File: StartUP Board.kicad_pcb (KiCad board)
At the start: 2 copper layers, 85.8 x 55 mm, 22 parts, among them IC1 AP7380-33W5-7, J1 Conn_01x05_Socket, U1 ANT13SECQE, U2 CD4049UBDR

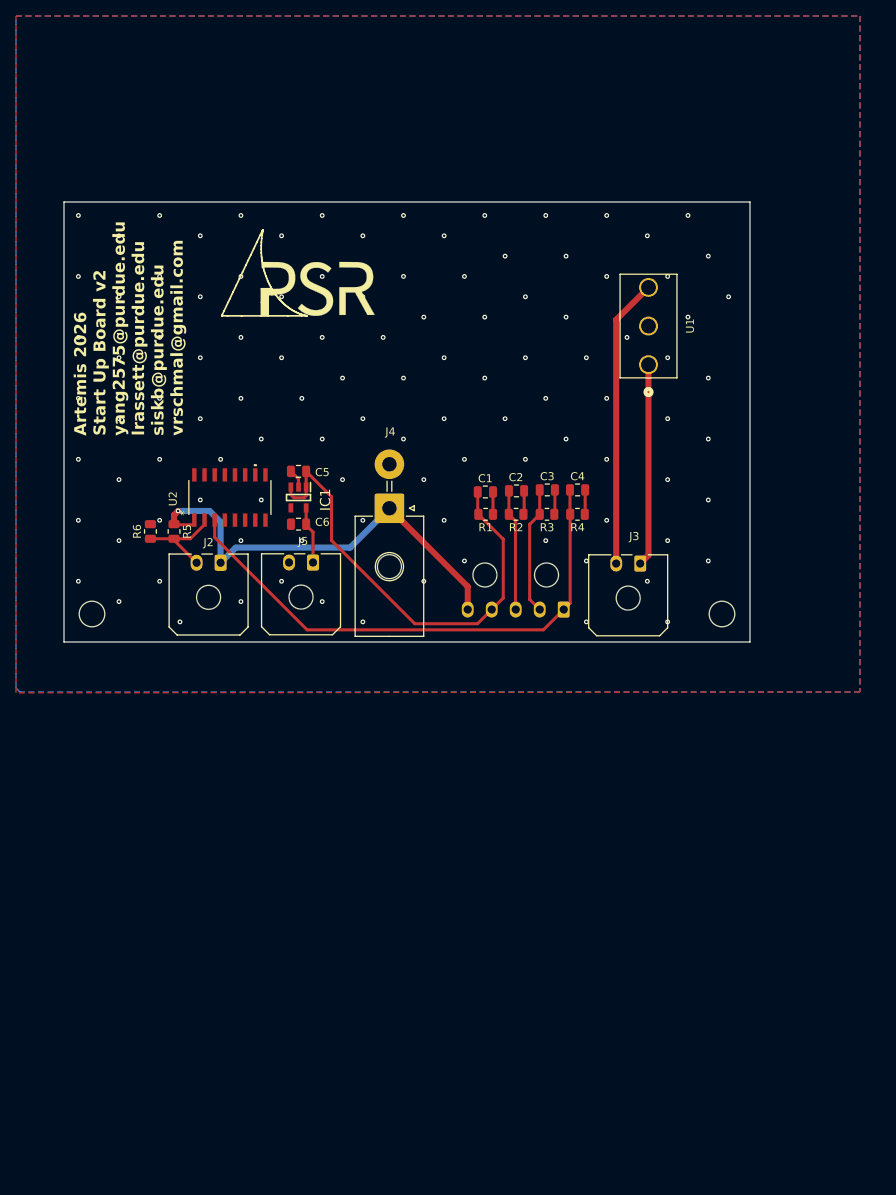
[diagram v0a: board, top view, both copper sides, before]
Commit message: furdue
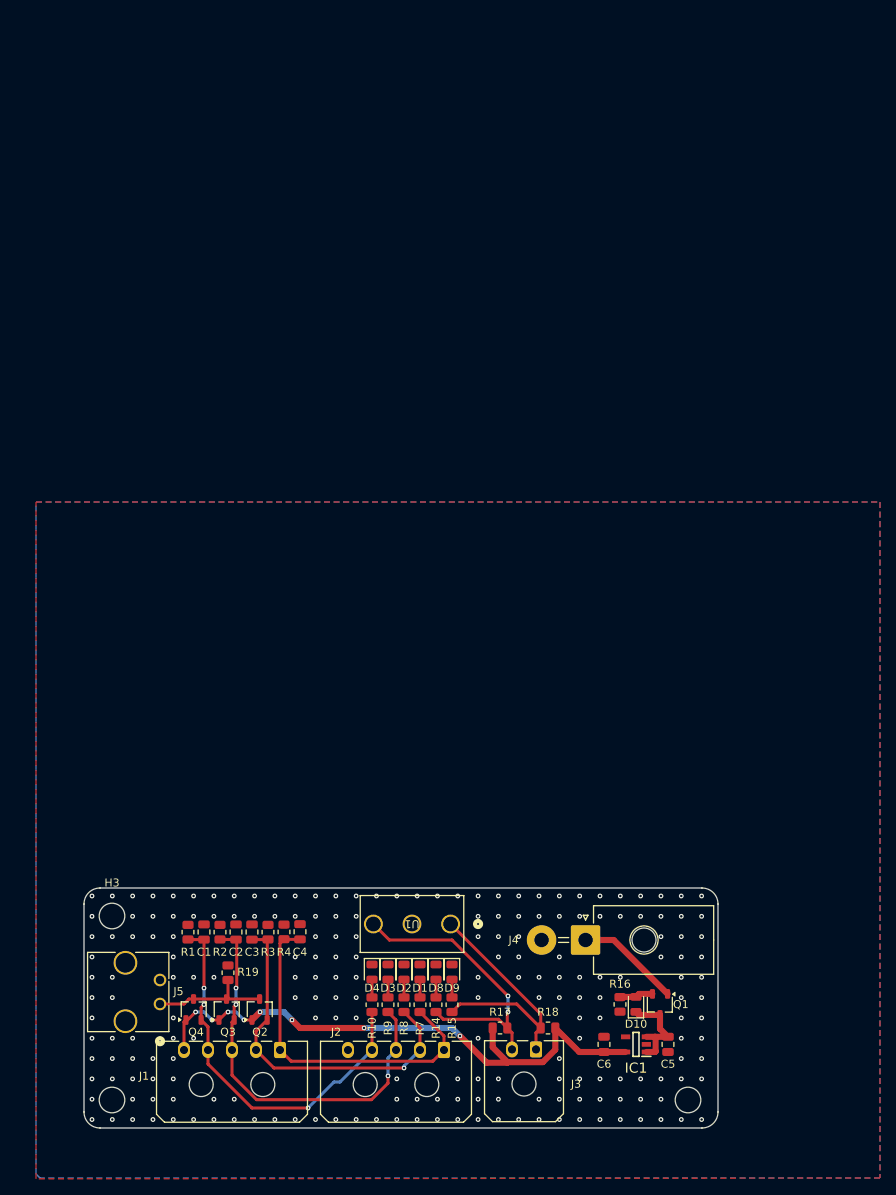
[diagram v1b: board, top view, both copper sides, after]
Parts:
- removed R5, R6: 100k, Resistor_SMD:R_0805_2012Metric
- removed U2: CD4049UBDR, CD4049UBDR:D16-M
- added D1: LED, LED_SMD:LED_0805_2012Metric, F.Cu at (166.0, 105.0)
- added D10: D_Zener, Diode_SMD:D_0805_2012Metric, F.Cu at (193.0, 109.0)
- added D2: LED, LED_SMD:LED_0805_2012Metric, F.Cu at (164.0, 105.0)
- added D3: LED, LED_SMD:LED_0805_2012Metric, F.Cu at (162.0, 105.0)
- added D4: LED, LED_SMD:LED_0805_2012Metric, F.Cu at (160.0, 105.0)
- added D8: LED, LED_SMD:LED_0805_2012Metric, F.Cu at (168.0, 105.0)
- added D9: LED, LED_SMD:LED_0805_2012Metric, F.Cu at (170.0, 105.0)
- added G***: LOGO, LOGO, B.Cu at (172.5, 106.0)
- added G***: LOGO, LOGO, B.Cu at (152.0, 107.5)
- added G***: LOGO, LOGO, B.Cu at (188.3, 108.1)
- added H3: MountingHole, MountingHole:MountingHole_3.2mm_M3, F.Cu at (127.5, 98.0)
- added Q1: PMOS, Package_TO_SOT_SMD:TSOT-23, F.Cu at (196.0, 109.0)
- added Q2: NMOS, Package_TO_SOT_SMD:TSOT-23, F.Cu at (145.9, 109.7)
- added Q3: NMOS, Package_TO_SOT_SMD:TSOT-23, F.Cu at (141.8, 109.7)
- added Q4: NMOS, Package_TO_SOT_SMD:TSOT-23, F.Cu at (137.7, 109.7)
- added R10: 680, Resistor_SMD:R_0805_2012Metric, F.Cu at (160.0, 109.1)
- added R14: 680, Resistor_SMD:R_0805_2012Metric, F.Cu at (168.0, 109.1)
- added R15: 680, Resistor_SMD:R_0805_2012Metric, F.Cu at (170.0, 109.1)
- added R16: 100k, Resistor_SMD:R_0805_2012Metric, F.Cu at (191.0, 109.0)
- added R17: 4.7k, Resistor_SMD:R_0805_2012Metric, F.Cu at (176.0, 112.0)
- added R18: 4.7k, Resistor_SMD:R_0805_2012Metric, F.Cu at (182.0, 112.0)
- added R19: 4.7k, Resistor_SMD:R_0805_2012Metric, F.Cu at (142.0, 105.1)
- added R7: 680, Resistor_SMD:R_0805_2012Metric, F.Cu at (166.0, 109.1)
- added R8: 680, Resistor_SMD:R_0805_2012Metric, F.Cu at (164.0, 109.1)
- added R9: 680, Resistor_SMD:R_0805_2012Metric, F.Cu at (162.0, 109.1)
- J1: moved to F.Cu
- J2: value ~ -> Conn_01x05_Socket; footprint Connector_Molex:Molex_Micro-Fit_3.0_43650-0200_1x02_P3.00mm_Horizontal -> Connector_Molex:Molex_Micro-Fit_3.0_43650-0500_1x05_P3.00mm_Horizontal
- J5: value ~ -> 436500204; footprint Connector_Molex:Molex_Micro-Fit_3.0_43650-0200_1x02_P3.00mm_Horizontal -> 1x2molex:CONN_SD-43650-002_02_MOL
- moved C5 85.2 mm to (197.0, 114.0), turned to -90 degrees
- moved IC1 80.3 mm to (193.0, 114.0), turned to 180 degrees
- moved C6 75.4 mm to (189.0, 114.0), turned to 90 degrees
- moved U1 74.2 mm to (169.8, 99.0), turned to 180 degrees
- moved J2 67.0 mm to (169.0, 114.8)
- moved C3 66.5 mm to (145.0, 100.0), turned to 90 degrees
- moved J1 65.5 mm to (148.5, 114.8)
- moved C2 65.3 mm to (143.0, 100.0), turned to 90 degrees
- moved C1 65.3 mm to (139.0, 100.0), turned to 90 degrees
- moved C4 65.2 mm to (151.0, 100.0), turned to 90 degrees
- moved R1 64.1 mm to (137.0, 100.0), turned to -90 degrees
- moved R2 64.0 mm to (141.0, 100.0), turned to -90 degrees
- moved R4 63.8 mm to (149.0, 100.0), turned to -90 degrees
- moved R3 62.8 mm to (147.0, 100.0), turned to -90 degrees
- moved J3 62.1 mm to (180.5, 114.7)
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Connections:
- C5 pad 1: /KEYSW_CHARGE -> +12V
- IC1 pad 1: /KEYSW_CHARGE -> +12V
- IC1 pad 3: /KEYSW_CHARGE -> +12V
- J1 pad 5: +12V -> +3.3V
- J2 pad 1: +12V -> /KEYSW_OFF
- J2 pad 2: /KeySwitch_LV -> /KEYSW_AUX
- J4 pad 1: +12V -> /AUX_IN
- J5 pad 1: +3.3V -> /CHARGE_MODE_LV
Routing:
- net +3.3V: track 7.18 -> 73.2 mm, vias 0 -> 8
- net +12V: track 56.7 -> 12.1 mm, vias 1 -> 0
- net /KEYSW_MAIN: track 15.2 -> 50.6 mm, vias 0 -> 3
- net /KEYSW_AUX: track 16.0 -> 44.5 mm, vias 0 -> 1
- net /KEYSW_OFF: track 67.5 -> 43.7 mm
- net /CHARGE_MODE_LV: track 0.00 -> 15.2 mm
- net GND: track 14.3 -> 0.00 mm, vias 108 -> 207
- net /AUX_IN: track 0.00 -> 13.0 mm
- net /KeySwitch_LV: track 12.2 -> 0.00 mm
- net /KEYSW_CHARGE: track 57.8 -> 48.6 mm, vias 0 -> 3
- net /FNR_REV: track 25.3 -> 33.3 mm
- net Net-(D10-A): track 0.00 -> 4.21 mm
- net Net-(D9-A): track 0.00 -> 2.24 mm
- net Net-(D8-A): track 0.00 -> 2.24 mm
- net Net-(D4-A): track 0.00 -> 2.24 mm
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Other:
- board size 85.8 x 55 mm -> 79.2 x 30 mm
- board text removed: "*"
